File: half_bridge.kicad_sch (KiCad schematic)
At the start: 36 parts, among them Q1 IGC025S08S1, Q2 IGC025S08S1, U16 SN74LVC1G66DCKR, U19 NCS2220AMUT1G, U4 AD8418, U5 LMG1205YFXR, U6 SN74LVC1G66DCKR

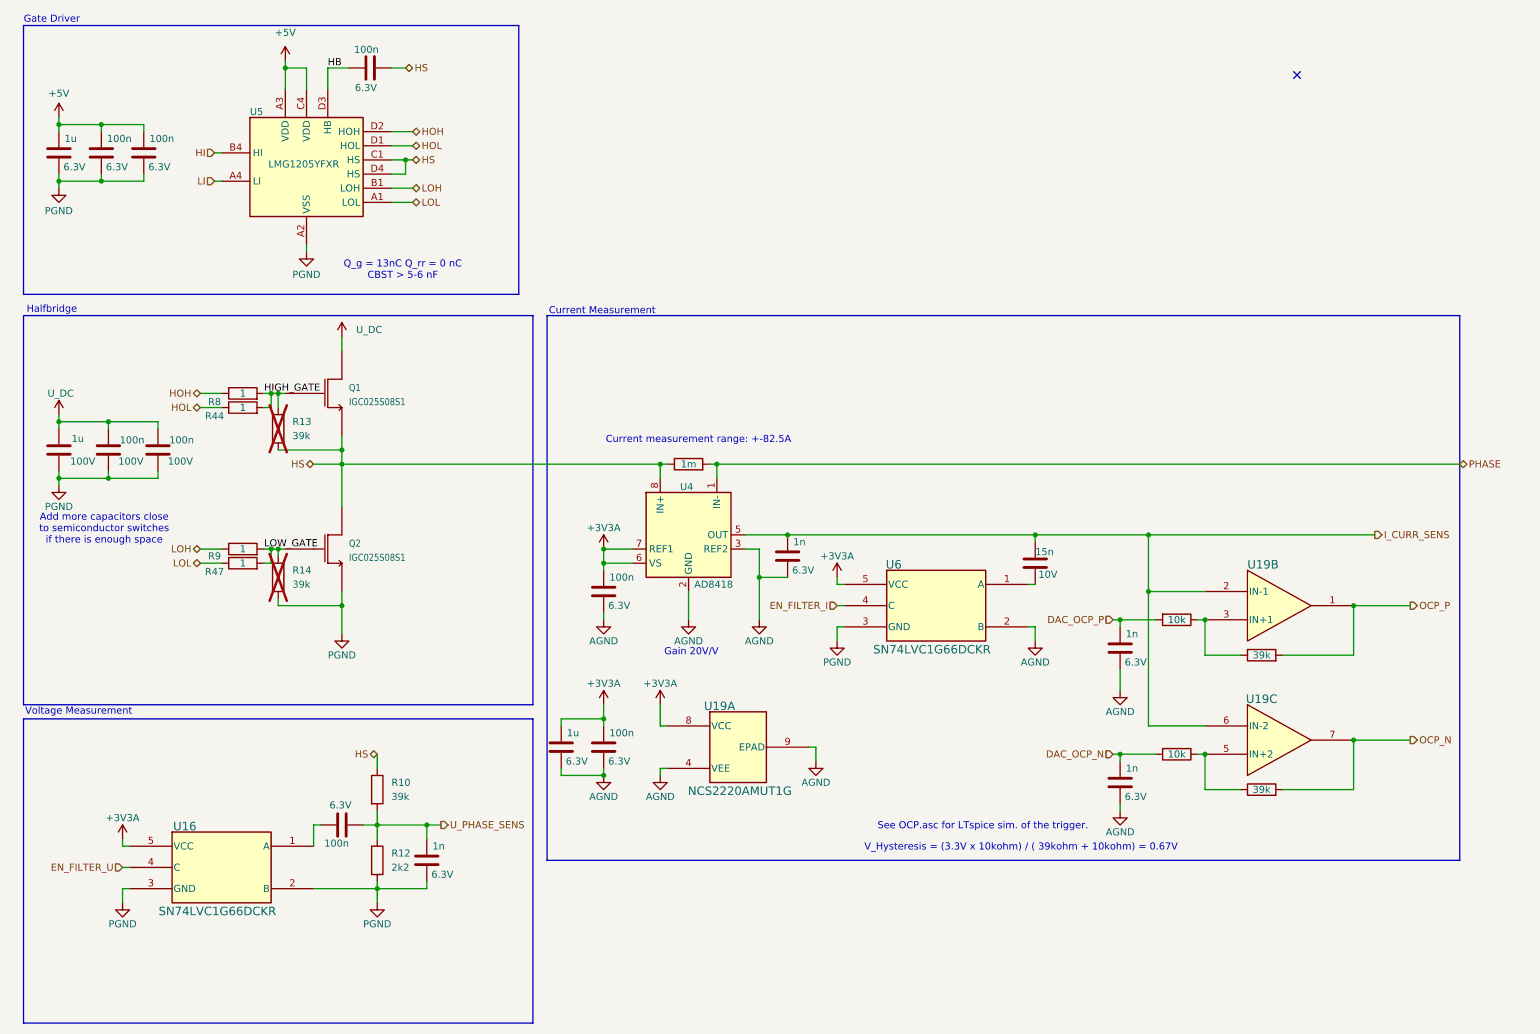
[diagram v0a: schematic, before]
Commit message: added the first draft of the layout
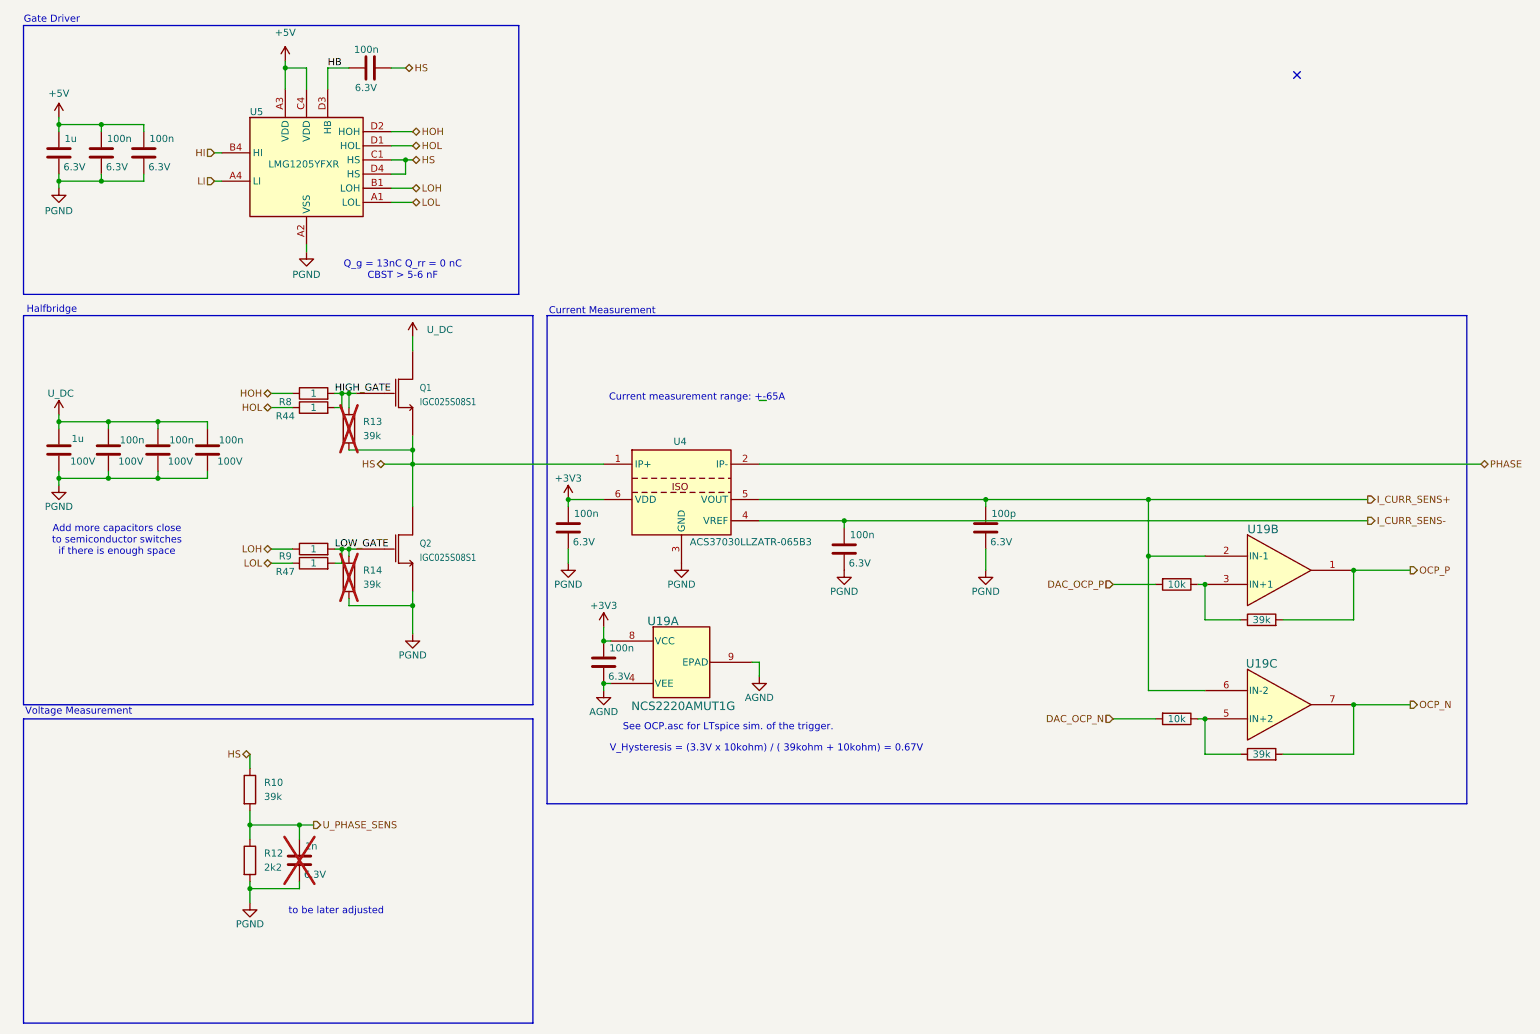
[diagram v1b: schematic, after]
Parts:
- removed C100: 1u, Capacitor_SMD:C_0402_1005Metric, symbol Device:C
- removed C101: 100n, Capacitor_SMD:C_0402_1005Metric, symbol Device:C
- removed C90: 15n, Capacitor_SMD:C_0402_1005Metric, symbol Device:C
- removed C94, C97: 1n, Capacitor_SMD:C_0201_0603Metric, symbol Device:C
- removed R11: 1m, NanoGaN:RES_00FEA_VIS-L, symbol Device:R
- removed U16, U6: SN74LVC1G66DCKR, NanoGaN:DCK5, symbol NanoGaN:SN74LVC1G66DCKR
- removed U4: AD8418, Package_SO:SOIC-8_3.9x4.9mm_P1.27mm, symbol Amplifier_Current:AD8418
- added C44: 100n, Capacitor_SMD:C_0805_2012Metric, symbol Device:C
- added C92: 100n, Capacitor_SMD:C_0402_1005Metric, symbol Device:C
- added U4: ACS37030LLZATR-065B3, ACS37030LLZATR020B3, symbol NanoGaN:ACS37030LLZATR-065B3
- C28: value 1n -> 100p; footprint Capacitor_SMD:C_0201_0603Metric -> Capacitor_SMD:C_0402_1005Metric; LCSC C541214 -> C1546
- C87: footprint Capacitor_SMD:C_0201_0603Metric -> Capacitor_SMD:C_0402_1005Metric; LCSC C541214 -> (none); now not fitted; now left out of the parts list
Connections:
- net AGND: now also C92.2; no longer C24.2, C28.2
- net HS: now also U4.1 (IP+)
- net PGND: now also C24.2, C25.2, C28.2, C44.2, U4.3 (GND)
- net PHASE: now also U4.2 (IP-)
- net U_DC: now also C44.1
- net U_PHASE_SENS: no longer C25.2
- net I_CURR_SENS-: now reaches C25.1
- net I_CURR_SENS-: now also U4.4 (VREF)
- net +3V3A renamed +3V3
- net +3V3: now also C92.1, U4.6 (VDD)
- net I_CURR_SENS renamed I_CURR_SENS+
- net I_CURR_SENS+: now also U4.5 (VOUT)
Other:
- note added: "Current measurement range: +-65A"
- note added: "to be later adjusted"
- note removed: "Current measurement range: +-82.5A"
- note removed: "Gain 20V/V"
- moved on the sheet: Q1, Q2, R10, R12, R13, R14, R44, R47, R8, R9, U19A, U19B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

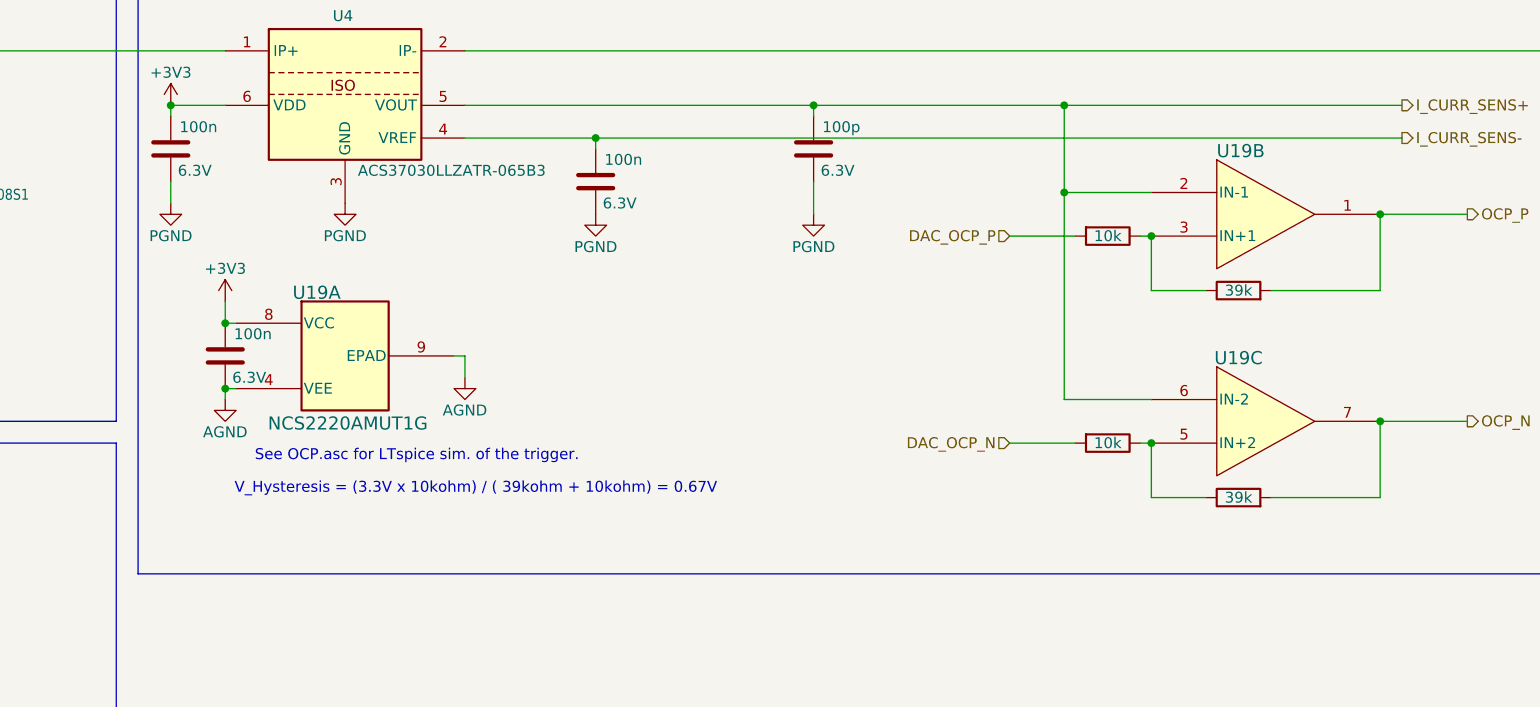
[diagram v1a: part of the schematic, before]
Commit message: wip layout
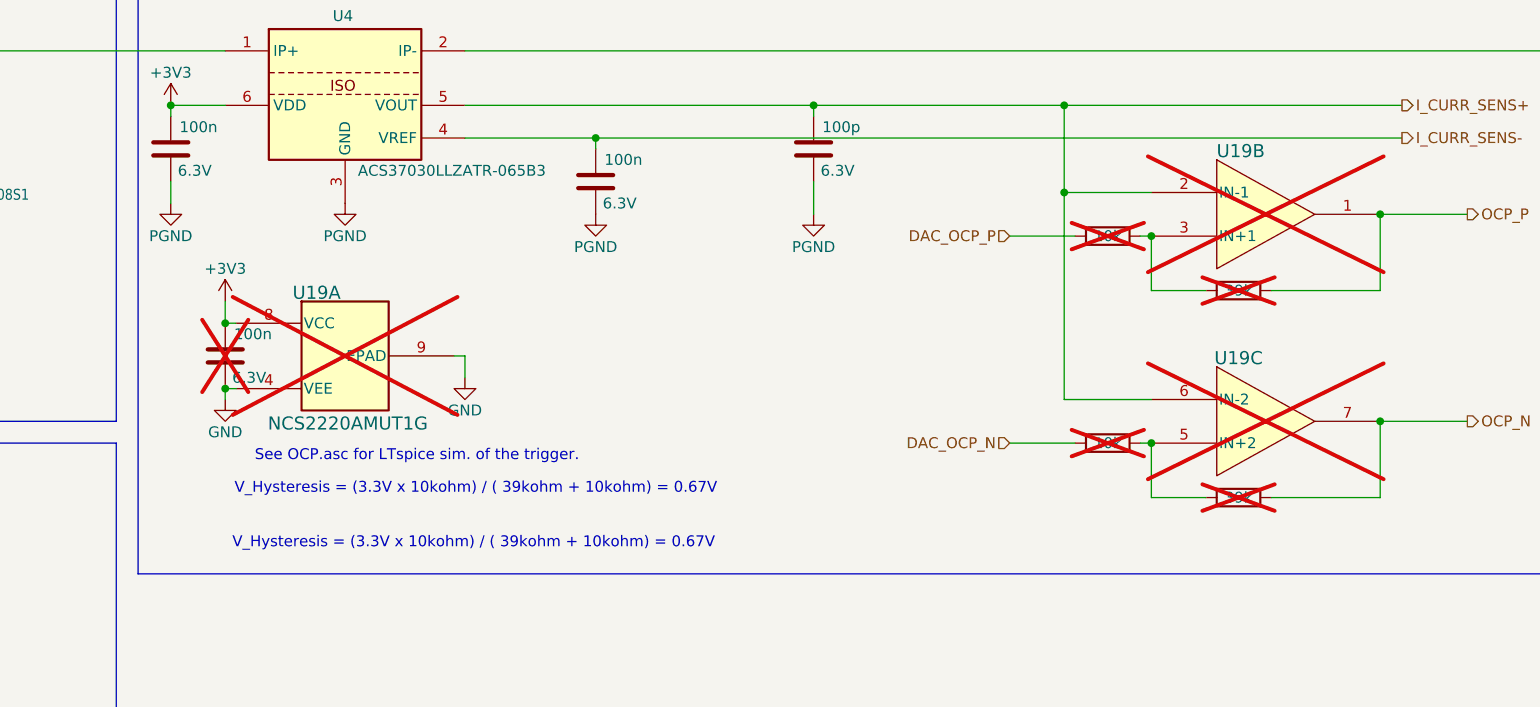
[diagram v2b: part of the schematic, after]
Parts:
- C24, C25: footprint Capacitor_SMD:C_0402_1005Metric -> Capacitor_SMD:C_0603_1608Metric_Pad1.08x0.95mm_HandSolder; LCSC C424821 -> (none)
- C28: footprint Capacitor_SMD:C_0402_1005Metric -> Capacitor_SMD:C_0603_1608Metric_Pad1.08x0.95mm_HandSolder; LCSC C1546 -> (none)
- C87: footprint Capacitor_SMD:C_0402_1005Metric -> Capacitor_SMD:C_0603_1608Metric_Pad1.08x0.95mm_HandSolder
- C92, R63, R66, R69, R72, U19: now not fitted; now left out of the parts list
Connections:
- net AGND renamed GND
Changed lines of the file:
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@@
 		)
 	)
+	(text "V_Hysteresis = (3.3V x 10kohm) / ( 39kohm + 10kohm) = 0.67V"
+		(exclude_from_sim no)
+		(at 145.796 151.384 0)
+		(effects
+			(font
+				(size 1.27 1.27)
+			)
+		)
+	)
 	(text "Gate Driver"
 		(exclude_from_sim no)
@@
 		(unit 1)
 		(exclude_from_sim no)
-		(in_bom yes)
-		(on_board yes)
-		(dnp no)
+		(in_bom no)
+		(on_board no)
+		(dnp yes)
 		(property "Reference" "R72"
 			(at 234.95 139.7 90)
@@
 			)
 		)
-		(property "Footprint" "Capacitor_SMD:C_0402_1005Metric"
+		(property "Footprint" "Capacitor_SMD:C_0603_1608Metric_Pad1.08x0.95mm_HandSolder"
 			(at 63.1952 168.91 0)
 			(effects
@@
 			)
 		)
-		(property "LCSC" ""
-			(at 62.23 165.1 0)
-			(effects
-				(font
-					(size 1.27 1.27)
-				)
-				(hide yes)
-			)
-		)
 		(property "Voltage Rating" "6.3V"
 			(at 65.024 167.64 0)
@@
 			)
 		)
-		(property "Value" "AGND"
+		(property "Value" "GND"
 			(at 116.84 138.43 0)
 			(effects
@@
 			)
 		)
-		(property "Footprint" "Capacitor_SMD:C_0402_1005Metric"
+		(property "Footprint" "Capacitor_SMD:C_0603_1608Metric_Pad1.08x0.95mm_HandSolder"
 			(at 160.9852 113.03 0)
 			(effects
@@
 			)
 		)
-		(property "Description" "100nF 6.3V X7R ±10% 0402 Multilayer Ceramic Capacitors MLCC - SMD/SMT ROHS"
-			(at 160.02 109.22 0)
-			(effects
-				(font
-					(size 1.27 1.27)
-				)
-				(hide yes)
-			)
-		)
-		(property "LCSC" "C424821"
+		(property "Description" "100nF 6.3V X7R ±10% 0603 Multilayer Ceramic Capacitors MLCC - SMD/SMT ROHS"
 			(at 160.02 109.22 0)
 			(effects
@@
 		(unit 1)
 		(exclude_from_sim no)
-		(in_bom yes)
-		(on_board yes)
-		(dnp no)
+		(in_bom no)
+		(on_board no)
+		(dnp yes)
 		(property "Reference" "R69"
 			(at 234.95 115.57 90)
@@
 		(unit 3)
 		(exclude_from_sim no)
-		(in_bom yes)
-		(on_board yes)
-		(dnp no)
+		(in_bom no)
+		(on_board no)
+		(dnp yes)
 		(property "Reference" "U19"
 			(at 234.95 129.794 0)
@@
 		(unit 2)
 		(exclude_from_sim no)
-		(in_bom yes)
-		(on_board yes)
-		(dnp no)
+		(in_bom no)
+		(on_board no)
+		(dnp yes)
 		(property "Reference" "U19"
 			(at 235.204 105.664 0)
@@
 			)
 		)
-		(property "Value" "AGND"
+		(property "Value" "GND"
 			(at 144.78 135.89 0)
 			(effects
@@
 		(unit 1)
 		(exclude_from_sim no)
-		(in_bom yes)
-		(on_board yes)
-		(dnp no)
+		(in_bom no)
+		(on_board no)
+		(dnp yes)
 		(property "Reference" "C92"
 			(at 119.38 128.27 0)
@@
 		(unit 1)
 		(exclude_from_sim no)
-		(in_bom yes)
-		(on_board yes)
-		(dnp no)
+		(in_bom no)
+		(on_board no)
+		(dnp yes)
 		(property "Reference" "R63"
 			(at 219.71 117.602 90)
@@
 		(unit 1)
 		(exclude_from_sim no)
-		(in_bom yes)
-		(on_board yes)
-		(dnp no)
+		(in_bom no)
+		(on_board no)
+		(dnp yes)
 		(property "Reference" "U19"
 			(at 130.302 122.174 0)
@@
 			)
 		)
-		(property "Footprint" "Capacitor_SMD:C_0402_1005Metric"
+		(property "Footprint" "Capacitor_SMD:C_0603_1608Metric_Pad1.08x0.95mm_HandSolder"
 			(at 186.3852 109.22 0)
 			(effects
@@
 			)
 		)
-		(property "Description" "100pF 50V C0G ±5% 0402 Multilayer Ceramic Capacitors MLCC - SMD/SMT ROHS"
-			(at 185.42 105.41 0)
-			(effects
-				(font
-					(size 1.27 1.27)
-				)
-				(hide yes)
-			)
-		)
-		(property "LCSC" "C1546"
+		(property "Description" "100pF 50V C0G ±5% 0603 Multilayer Ceramic Capacitors MLCC - SMD/SMT ROHS"
 			(at 185.42 105.41 0)
 			(effects
@@
 			)
 		)
-		(property "Footprint" "Capacitor_SMD:C_0402_1005Metric"
+		(property "Footprint" "Capacitor_SMD:C_0603_1608Metric_Pad1.08x0.95mm_HandSolder"
 			(at 111.4552 109.22 0)
 			(effects
@@
 			)
 		)
-		(property "Description" "100nF 6.3V X7R ±10% 0402 Multilayer Ceramic Capacitors MLCC - SMD/SMT ROHS"
-			(at 110.49 105.41 0)
-			(effects
-				(font
-					(size 1.27 1.27)
-				)
-				(hide yes)
-			)
-		)
-		(property "LCSC" "C424821"
+		(property "Description" "100nF 6.3V X7R ±10% Multilayer Ceramic Capacitors MLCC - SMD/SMT ROHS"
 			(at 110.49 105.41 0)
 			(effects
@@
 		(unit 1)
 		(exclude_from_sim no)
-		(in_bom yes)
-		(on_board yes)
-		(dnp no)
+		(in_bom no)
+		(on_board no)
+		(dnp yes)
 		(property "Reference" "R66"
 			(at 219.71 141.732 90)
